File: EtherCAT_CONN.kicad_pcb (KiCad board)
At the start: 2 copper layers, 21 x 27 mm, 28 parts, among them CN1 5019530507, CN2 5019530507, J2 Conn_01x12, U1 SRV05-4, U2 SRV05-4

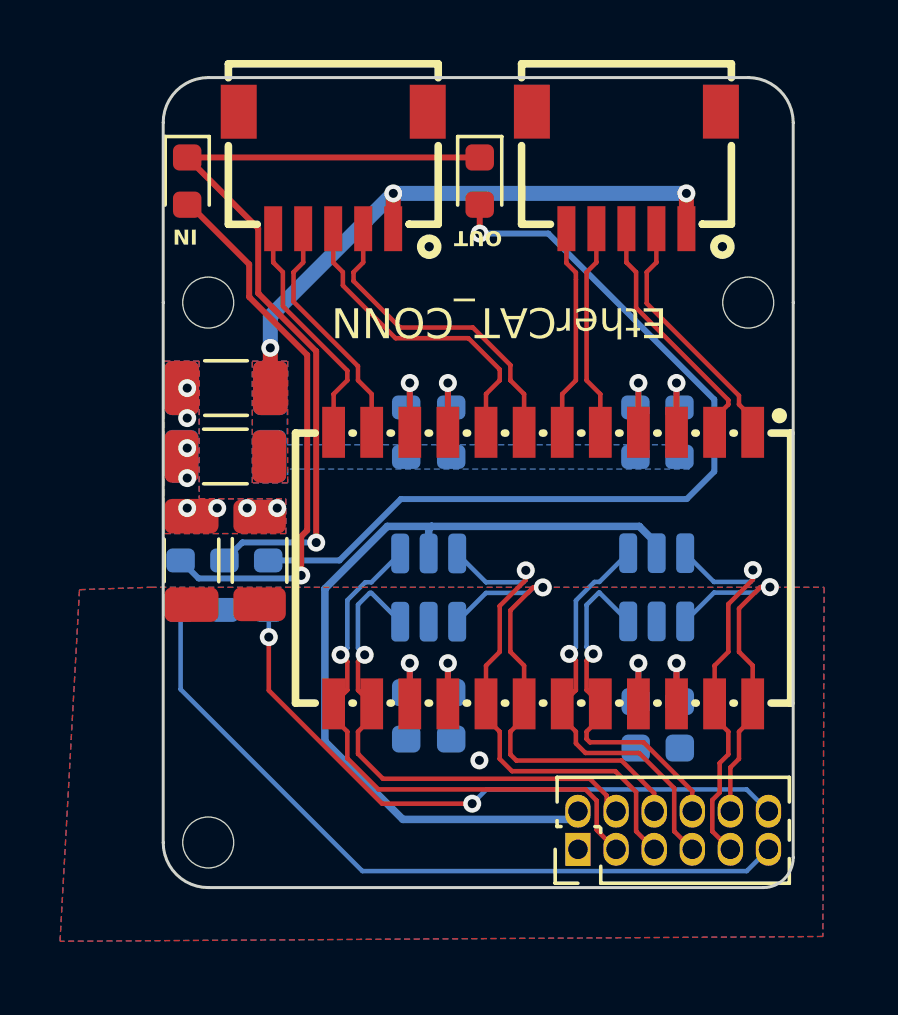
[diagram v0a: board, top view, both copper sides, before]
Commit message: Official version
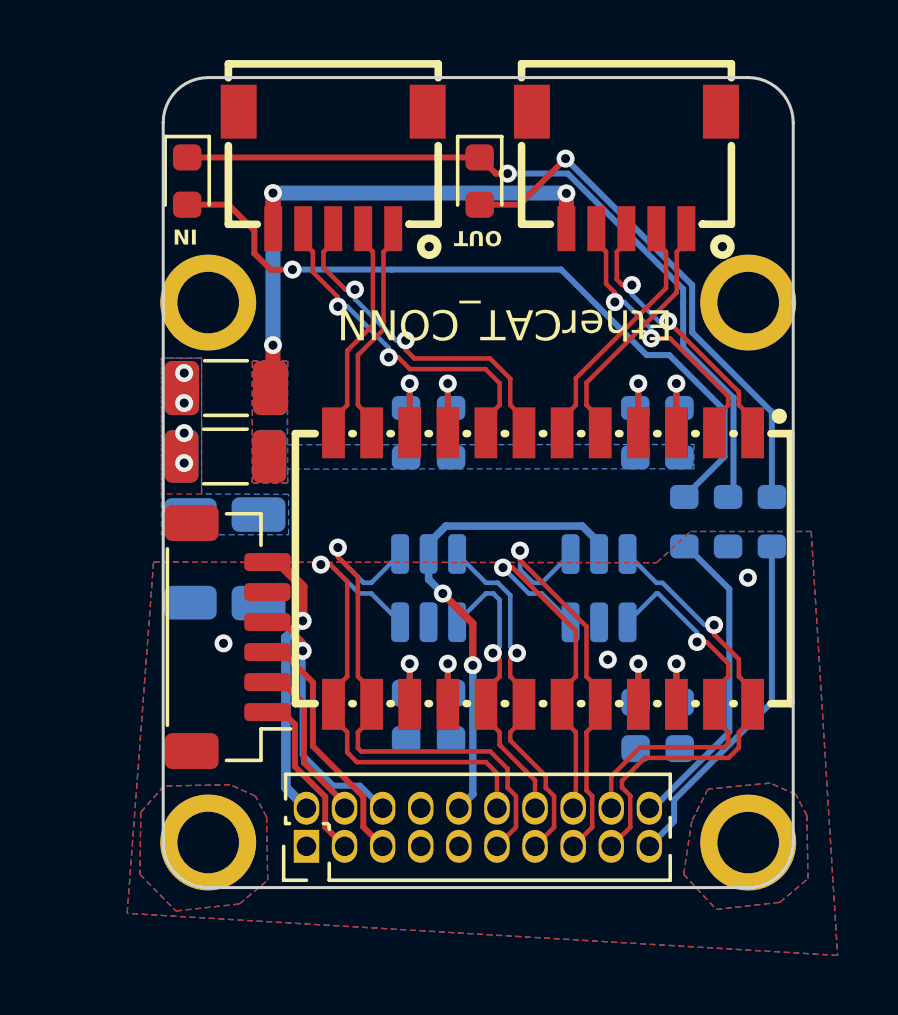
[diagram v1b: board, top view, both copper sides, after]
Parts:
- added H4: MountingHole, EXTRA IC:M1.6, F.Cu at (165.7, 106.2)
- added J1: Conn_01x20, Connector_PinHeader_1.27mm:ECAT_20pin, F.Cu at (156.7, 105.6)
- C5, R1: moved to B.Cu
- H1, H2, H3: footprint EXTRA IC:MountingHole_1.7mm_M1.6 -> EXTRA IC:M1.6
- J2: value Conn_01x12 -> Conn_01x06; footprint Connector_PinHeader_1.27mm:ECAT -> Connector_JST:JST_SH_BM06B-SRSS-TB_1x06-1MP_P1.00mm_Vertical
- moved R9 16.9 mm to (166.5, 95.5)
- moved R10 16.9 mm to (165.0, 95.5)
- moved R8 16.9 mm to (163.6, 95.5)
- moved J2 16.2 mm to (148.3, 99.3)
- moved R1 2.30 mm to (147.1, 96.7)
- moved C5 2.24 mm to (149.4, 96.7)
- moved U1 1.92 mm to (160.7, 97.7)
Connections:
- J2 pad 1: GND -> /SWCLK
- J2 pad 2: A3V3 -> /SWDIO
- J2 pad 3: /CONN/P1_TXOP -> /USART_RX
- J2 pad 4: /CONN/P1_TXON -> /USART_TX
- J2 pad 5: /CONN/P1_RXIP -> GND
- J2 pad 6: /CONN/P1_RXIN -> +5V
- L1 pad 1: /CONN/P0_MRXIN -> /CONN/P0_MRXIP
- L1 pad 11: /CONN/P1_MTXON -> /CONN/P1_MTXOP
- L1 pad 12: /CONN/P1_MTXOP -> /CONN/P1_MTXON
- L1 pad 13: /CONN/P1_TXOP -> /CONN/P1_TXON
- L1 pad 14: /CONN/P1_TXON -> /CONN/P1_TXOP
- L1 pad 17: /CONN/P1_RXIP -> /CONN/P1_RXIN
- L1 pad 18: /CONN/P1_RXIN -> /CONN/P1_RXIP
- L1 pad 19: /CONN/P0_TXOP -> /CONN/P0_TXON
- L1 pad 2: /CONN/P0_MRXIP -> /CONN/P0_MRXIN
- L1 pad 20: /CONN/P0_TXON -> /CONN/P0_TXOP
- L1 pad 23: /CONN/P0_RXIP -> /CONN/P0_RXIN
- L1 pad 24: /CONN/P0_RXIN -> /CONN/P0_RXIP
- L1 pad 5: /CONN/P0_MTXON -> /CONN/P0_MTXOP
- L1 pad 6: /CONN/P0_MTXOP -> /CONN/P0_MTXON
- L1 pad 7: /CONN/P1_MRXIN -> /CONN/P1_MRXIP
- L1 pad 8: /CONN/P1_MRXIP -> /CONN/P1_MRXIN
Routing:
- net /CONN/P0_ACT: track 25.1 -> 10.6 mm
- net A3V3: track 28.1 -> 16.2 mm, vias 0 -> 2
- net Net-(D2-A): track 29.6 -> 17.6 mm
- net /CONN/P1_ACT: track 21.4 -> 11.7 mm, vias 2 -> 0
- net +5V: track 0.00 -> 9.42 mm, vias 0 -> 1
- net /USART_TX: track 0.00 -> 8.61 mm, vias 0 -> 1
- net /USART_RX: track 0.00 -> 8.36 mm
- net /CONN/P1_RXIN: track 15.8 -> 9.43 mm
- net Net-(D1-A): track 18.5 -> 24.6 mm
- net /SWCLK: track 0.00 -> 5.84 mm
- net /SWDIO: track 0.00 -> 5.56 mm
- net /CONN/P1_RXIP: track 17.2 -> 11.7 mm
- net /CONN/P0_RXIP: track 13.5 -> 15.6 mm
- net Net-(D1-K): track 27.7 -> 26.1 mm
- net Net-(C7-Pad2): track 20.3 -> 18.7 mm
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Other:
- outline, holes or cut-outs redrawn
